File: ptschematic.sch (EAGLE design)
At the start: 26 parts, among them U3 NCP1117LPST33T3G, U4 BGM13S, Y2 32MHz

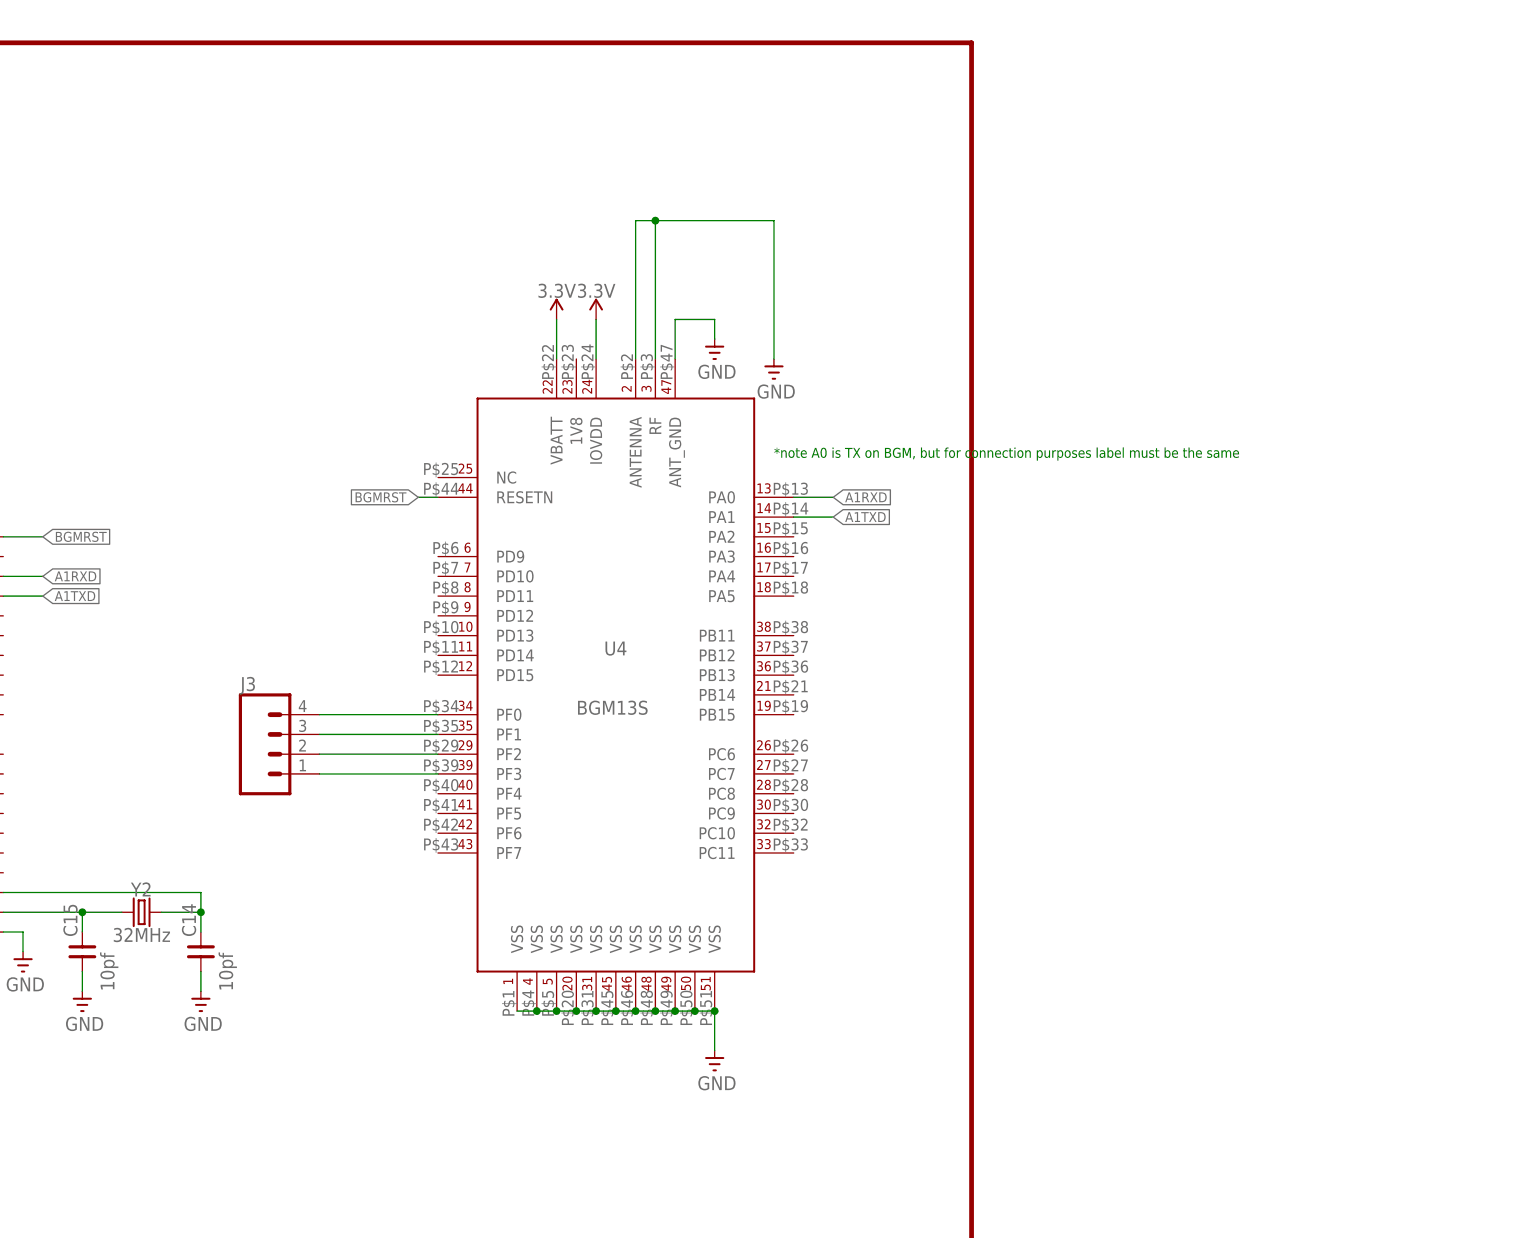
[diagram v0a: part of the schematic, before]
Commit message: Final Board and Gerber files
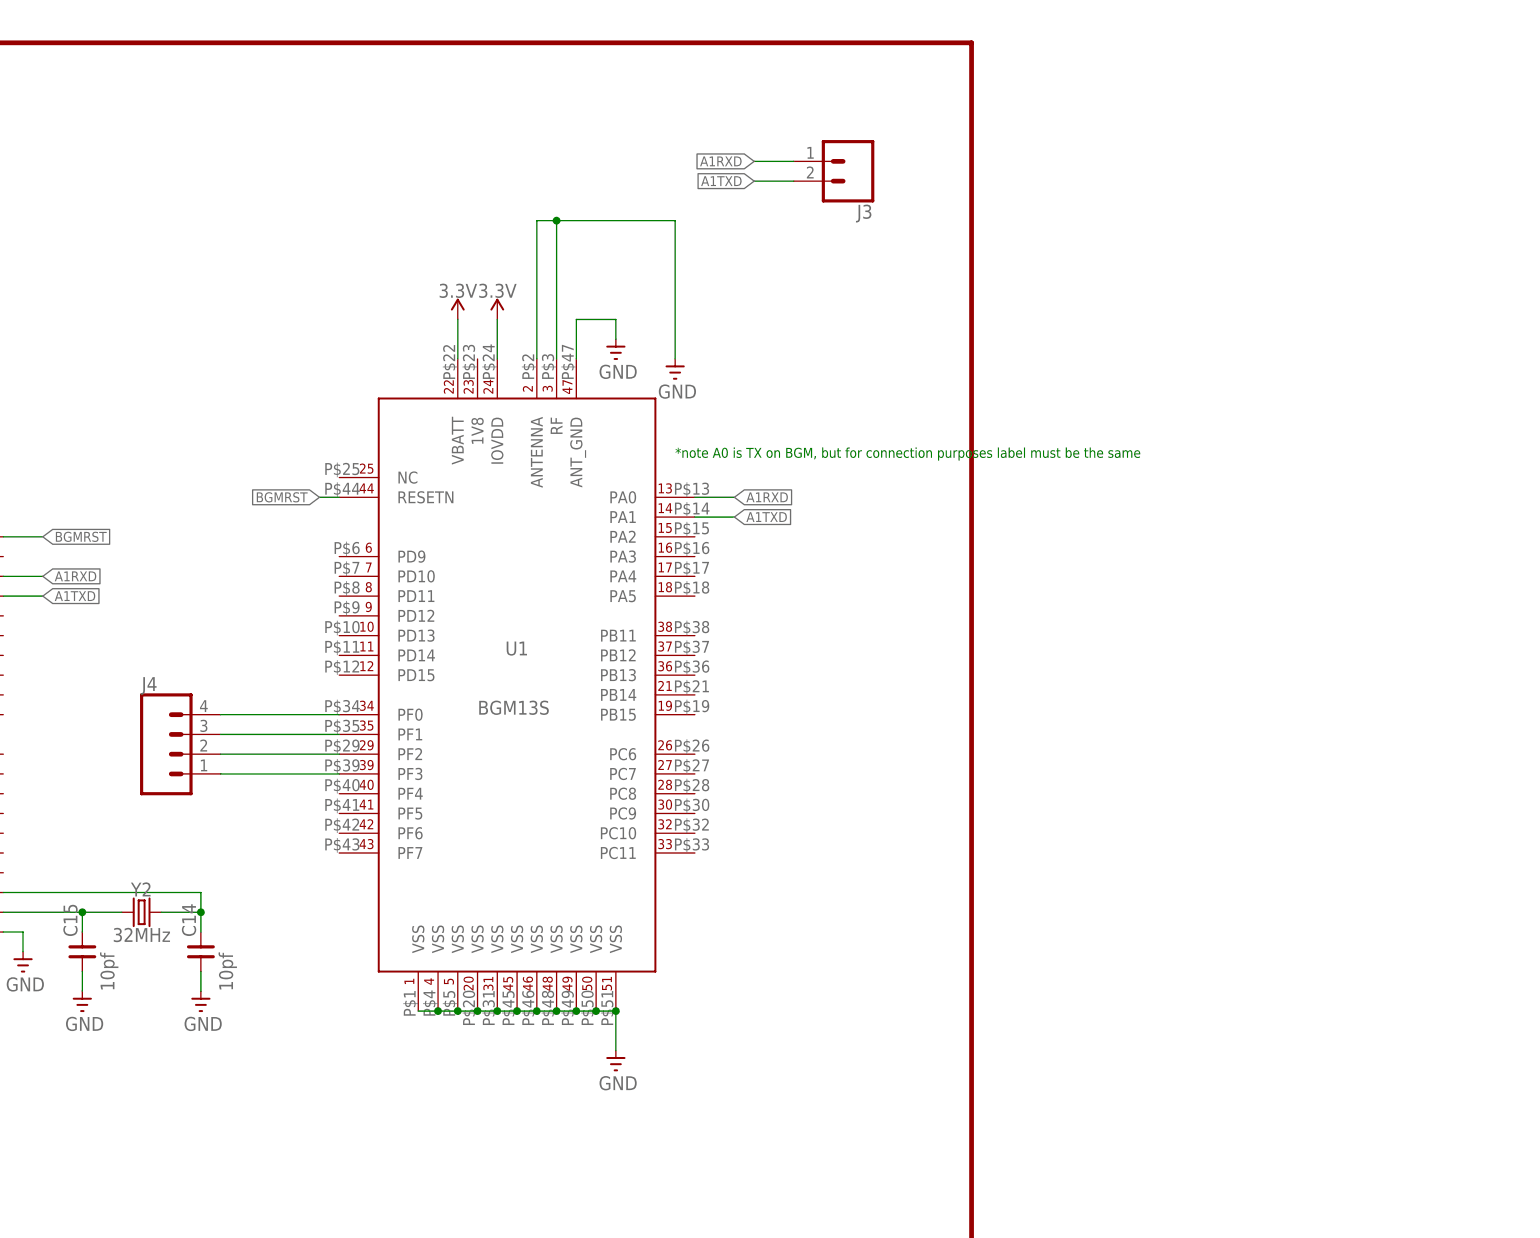
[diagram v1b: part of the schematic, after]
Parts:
- removed U4: BGM13S, BMES-Spr2019:BGM13S
- added J4: (no value), SparkFun-Connectors:CONN_04
- added U1: BGM13S, BMES-Spr2019:BGM13S
- J3: device SparkFun-Connectors:CONN_04 -> SparkFun-Connectors:CONN_02
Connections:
- removed net N$1: J3.4, U4.PF0
- removed net N$2: J3.3, U4.PF1
- removed net N$3: J3.2, U4.PF2
- removed net N$4: J3.1, U4.PF3
- new net N$5: J4.4, U1.PF0
- new net N$6: J4.3, U1.PF1
- new net N$7: J4.2, U1.PF2
- new net N$8: J4.1, U1.PF3
- net 3.3V: now also U1.IOVDD, U1.VBATT; no longer U4.IOVDD, U4.VBATT
- net A1RXD: now also J3.1, U1.PA0; no longer U4.PA0
- net A1TXD: now also J3.2, U1.PA1; no longer U4.PA1
- net BGMRST: now also U1.RESETN; no longer U4.RESETN
- net GND: now also U1.ANTENNA, U1.ANT_GND, U1.RF, U1.VSS@1, U1.VSS@10, U1.VSS@11, U1.VSS@2, U1.VSS@3, U1.VSS@4, U1.VSS@5, U1.VSS@6, U1.VSS@7, U1.VSS@8, U1.VSS@9; no longer U4.ANTENNA, U4.ANT_GND, U4.RF, U4.VSS@1, U4.VSS@10, U4.VSS@11, U4.VSS@2, U4.VSS@3, U4.VSS@4, U4.VSS@5, U4.VSS@6, U4.VSS@7, U4.VSS@8, U4.VSS@9
